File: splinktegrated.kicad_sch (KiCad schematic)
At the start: 51 parts, among them J1 USB_C_Receptacle_USB2.0, J10 Ribbon, J11 RJ9, J12 Conn_01x04_Female, J13 Conn_01x02_Female, J14 USB_C_Receptacle_USB2.0, J2 Conn_01x04_Female, J3 Conn_01x04_Female, J4 Conn_01x04_Female, J5 Conn_01x02, J6 RJ9, J7 trackball, J8 Ribbon, J9 RGB, SW1 SW_SPST, SW2 SW_SPST, U1 RP2040, U2 USBLC6-2P6, U3 XC6210B332MR-G, U4 USBLC6-2P6, U5 W25Q128JVS, Y1 Crystal_GND24

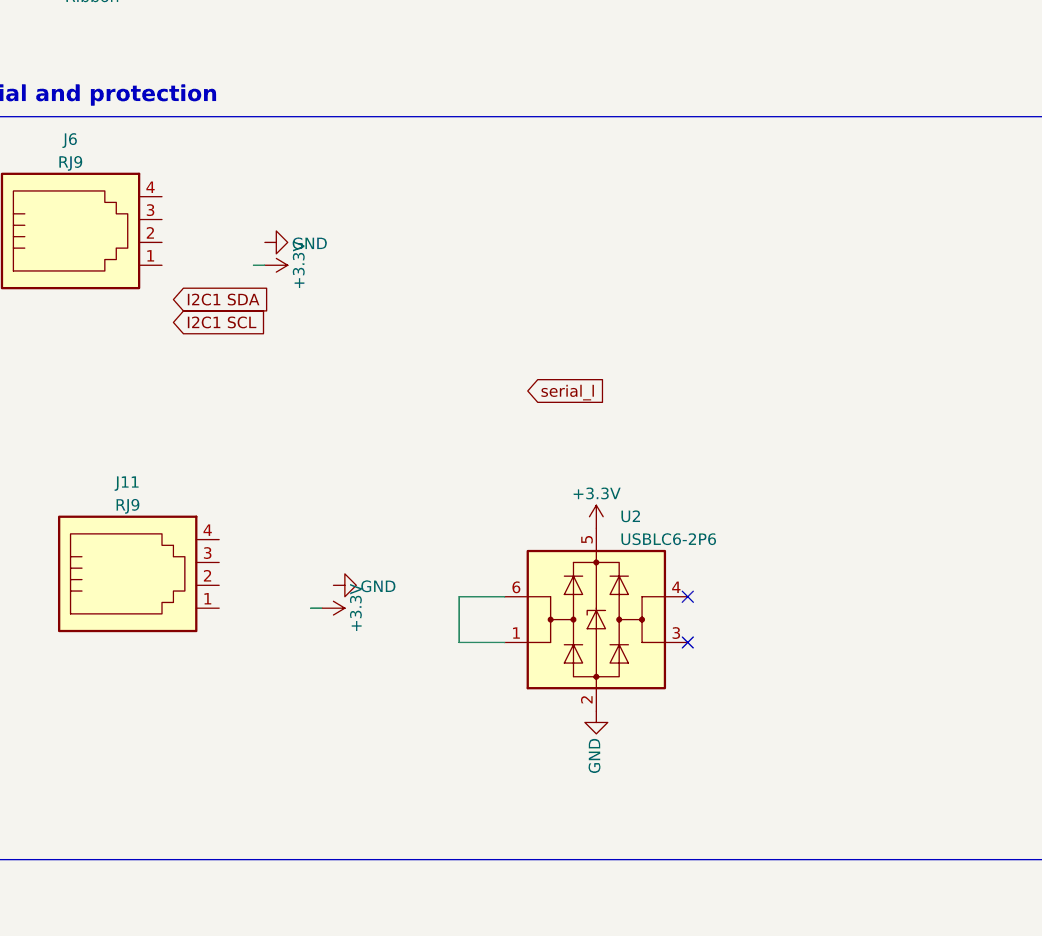
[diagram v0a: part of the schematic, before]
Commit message: minor changes
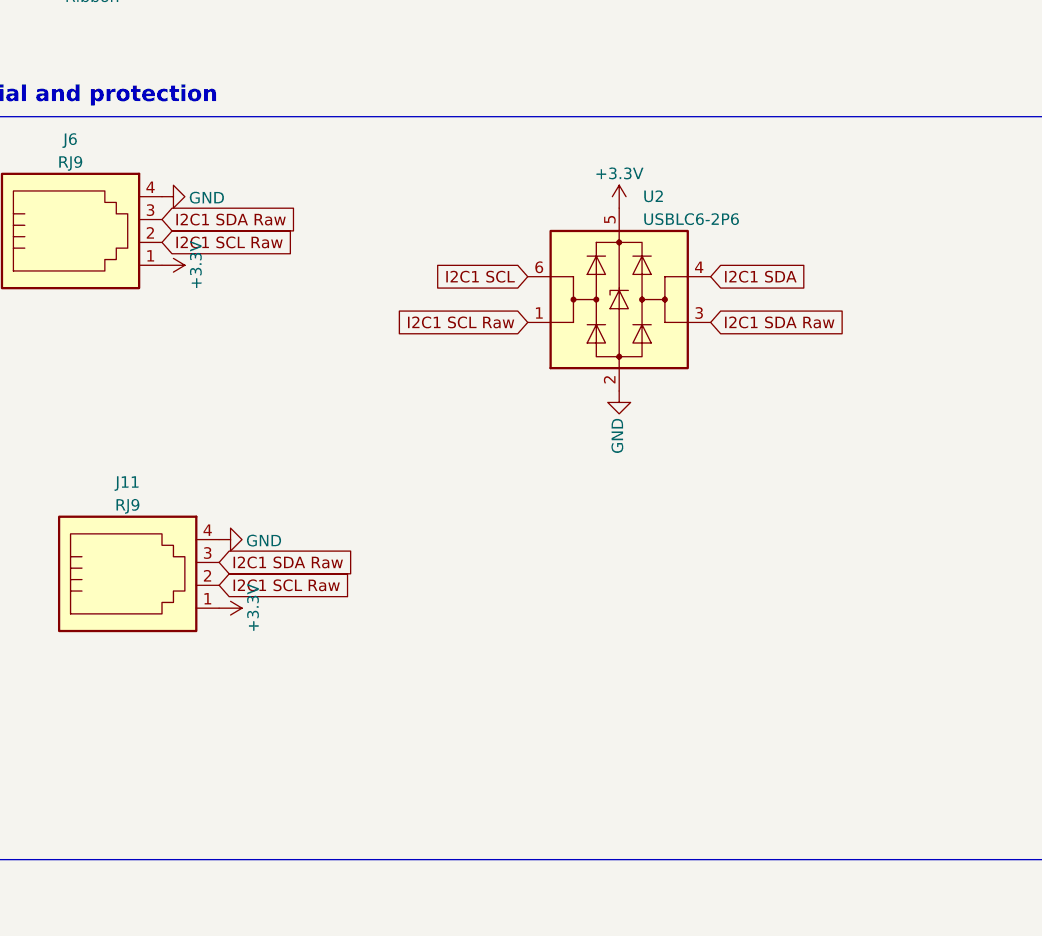
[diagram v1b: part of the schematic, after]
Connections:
- net +3V3: now also J11.1, J6.1
- net GND: now also J11.4, J6.4
- net I2C1 SCL: now also U2.6 (I/O1)
- net I2C1 SDA: now also U2.4 (I/O2)
- net I2C1 SCL Raw: now reaches J11.2
- net I2C1 SCL Raw: now also J6.2, U2.1 (I/O1)
- net I2C1 SDA Raw: now reaches J11.3
- net I2C1 SDA Raw: now also J6.3, U2.3 (I/O2)
- no-connect marks 14 -> 12
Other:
- moved on the sheet: U2

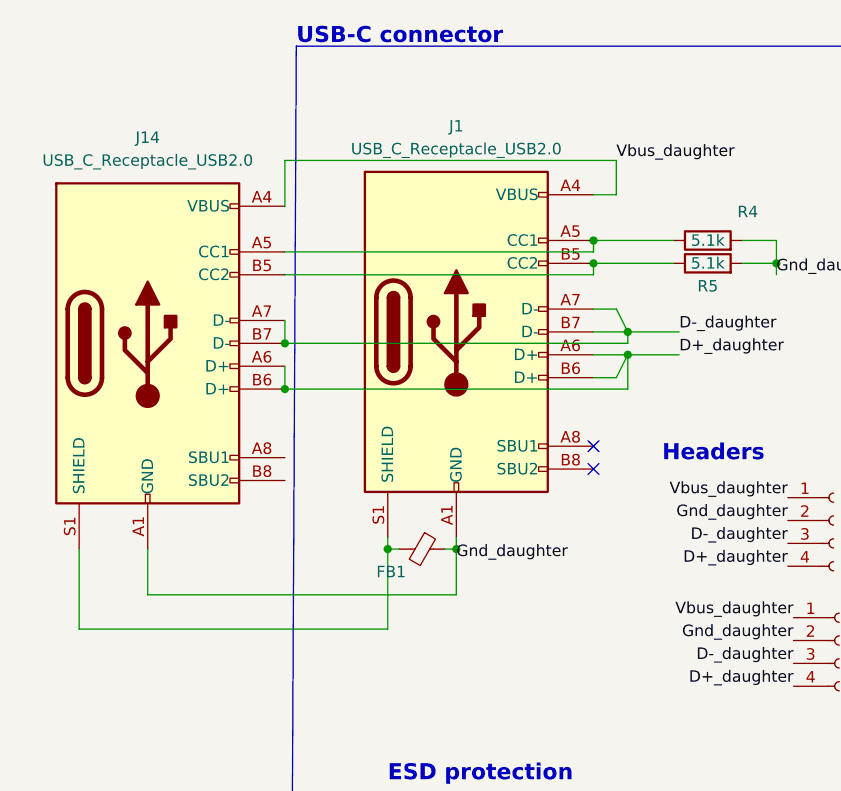
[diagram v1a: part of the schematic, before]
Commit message: major work done. outline finished
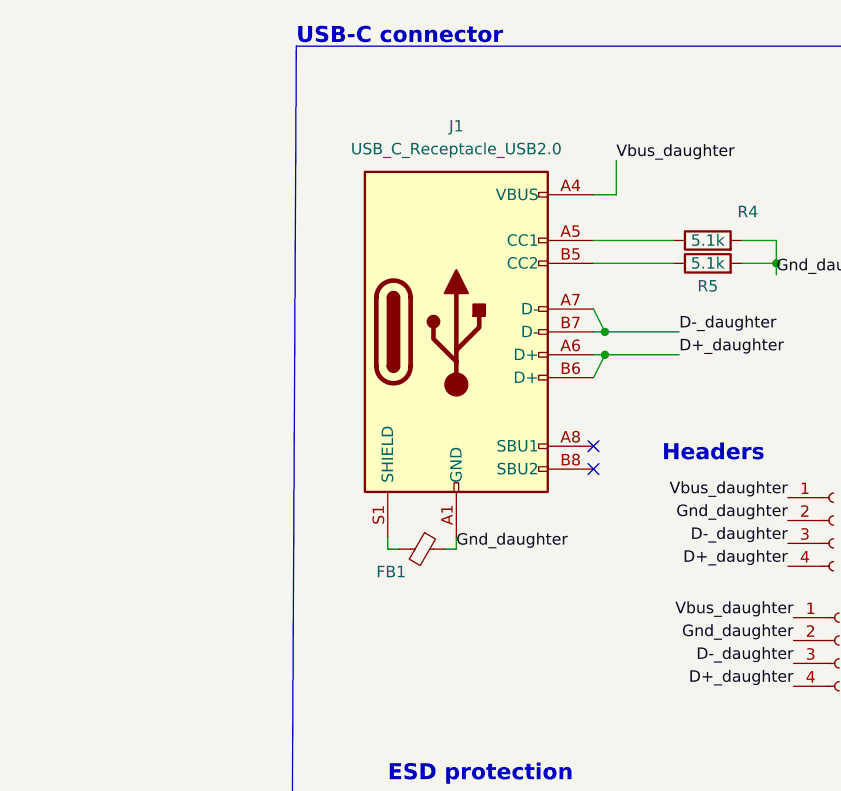
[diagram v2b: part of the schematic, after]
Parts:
- removed J14: USB_C_Receptacle_USB2.0, Connector_USB:USB_C_Receptacle_HRO_TYPE-C-31-M-12, symbol Connector:USB_C_Receptacle_USB2.0
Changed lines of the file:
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@@
     (company "bastardkb")
   )
-  (junction (at -123.19 54.61) (diameter 0) (color 0 0 0 0)
-  )
   (junction (at 46.99 127) (diameter 0) (color 0 0 0 0)
   )
@@
   (junction (at 154.94 38.1) (diameter 0) (color 0 0 0 0)
   )
+  (junction (at -87.63 50.8) (diameter 0) (color 0 0 0 0)
+  )
   (junction (at 162.56 38.1) (diameter 0) (color 0 0 0 0)
   )
@@
   (junction (at 40.005 172.72) (diameter 0) (color 0 0 0 0)
   )
-  (junction (at -85.09 48.26) (diameter 0) (color 0 0 0 0)
-  )
-  (junction (at -111.76 72.39) (diameter 0) (color 0 0 0 0)
-  )
   (junction (at 157.48 38.1) (diameter 0) (color 0 0 0 0)
   )
@@
   (junction (at 160.02 38.1) (diameter 0) (color 0 0 0 0)
   )
+  (junction (at -87.63 48.26) (diameter 0) (color 0 0 0 0)
+  )
   (junction (at 33.02 113.03) (diameter 0) (color 0 0 0 0)
   )
@@
   (junction (at 154.94 144.78) (diameter 0) (color 0 0 0 0)
   )
-  (junction (at -104.14 72.39) (diameter 0) (color 0 0 0 0)
-  )
   (junction (at 198.12 106.68) (diameter 0) (color 0 0 0 0)
   )
@@
   (junction (at -68.58 40.64) (diameter 0) (color 0 0 0 0)
   )
-  (junction (at -123.19 49.53) (diameter 0) (color 0 0 0 0)
-  )
   (junction (at 130.81 185.42) (diameter 0) (color 0 0 0 0)
   )
   (junction (at 97.79 106.68) (diameter 0) (color 0 0 0 0)
   )
-  (junction (at -88.9 38.1) (diameter 0) (color 0 0 0 0)
-  )
   (junction (at 33.02 115.57) (diameter 0) (color 0 0 0 0)
   )
-  (junction (at -85.09 50.8) (diameter 0) (color 0 0 0 0)
-  )
   (junction (at 243.84 119.38) (diameter 0) (color 0 0 0 0)
   )
   (junction (at 29.845 29.845) (diameter 0) (color 0 0 0 0)
-  )
-  (junction (at -88.9 40.64) (diameter 0) (color 0 0 0 0)
   )
   (junction (at 143.51 38.1) (diameter 0) (color 0 0 0 0)
@@
     (stroke (width 0) (type default))
   )
-  (wire (pts (xy -123.19 49.53) (xy -85.09 49.53))
-    (stroke (width 0) (type default))
-  )
-  (wire (pts (xy -123.19 41.91) (xy -88.9 41.91))
-    (stroke (width 0) (type default))
-  )
   (wire (pts (xy 101.6 175.26) (xy 110.49 175.26))
     (stroke (width 0) (type default))
@@
     (stroke (width 0) (type default))
   )
-  (wire (pts (xy -111.76 81.28) (xy -111.76 72.39))
-    (stroke (width 0) (type default))
-  )
-  (wire (pts (xy -88.9 50.8) (xy -85.09 50.8))
+  (wire (pts (xy -88.9 50.8) (xy -87.63 50.8))
     (stroke (width 0) (type default))
   )
@@
     (stroke (width 0) (type default))
   )
-  (wire (pts (xy -85.09 54.61) (xy -85.09 50.8))
-    (stroke (width 0) (type default))
-  )
   (wire (pts (xy 267.97 137.16) (xy 256.54 137.16))
     (stroke (width 0) (type default))
@@
     (stroke (width 0) (type default))
   )
-  (wire (pts (xy -138.43 72.39) (xy -138.43 77.47))
-    (stroke (width 0) (type default))
-  )
   (wire (pts (xy 48.895 29.845) (xy 52.705 29.845))
     (stroke (width 0) (type default))
@@
     (stroke (width 0) (type default))
   )
-  (wire (pts (xy -88.9 39.37) (xy -88.9 38.1))
-    (stroke (width 0) (type default))
-  )
-  (wire (pts (xy -85.09 48.26) (xy -88.9 48.26))
-    (stroke (width 0) (type default))
-  )
   (polyline (pts (xy -39.37 137.795) (xy -121.92 137.795))
     (stroke (width 0) (type default))
@@
     (stroke (width 0) (type default))
   )
-  (wire (pts (xy -88.9 45.72) (xy -86.36 45.72))
-    (stroke (width 0) (type default))
-  )
   (wire (pts (xy 93.98 90.17) (xy 93.98 104.14))
     (stroke (width 0) (type default))
@@
     (stroke (width 0) (type default))
   )
-  (wire (pts (xy -86.36 45.72) (xy -85.09 48.26))
+  (wire (pts (xy -88.9 45.72) (xy -87.63 48.26))
     (stroke (width 0) (type default))
   )
@@
     (stroke (width 0) (type default))
   )
-  (wire (pts (xy -123.19 29.21) (xy -86.36 29.21))
-    (stroke (width 0) (type default))
-  )
   (wire (pts (xy 182.88 109.22) (xy 191.77 109.22))
     (stroke (width 0) (type default))
@@
     (stroke (width 0) (type default))
   )
-  (wire (pts (xy -85.09 49.53) (xy -85.09 48.26))
-    (stroke (width 0) (type default))
-  )
   (wire (pts (xy 175.26 40.64) (xy 175.26 38.1))
     (stroke (width 0) (type default))
   )
-  (wire (pts (xy -146.05 72.39) (xy -146.05 81.28))
+  (wire (pts (xy -87.63 48.26) (xy -88.9 48.26))
     (stroke (width 0) (type default))
   )
@@
     (stroke (width 0) (type default))
   )
-  (wire (pts (xy -88.9 41.91) (xy -88.9 40.64))
-    (stroke (width 0) (type default))
-  )
   (wire (pts (xy 58.42 113.03) (xy 58.42 118.11))
     (stroke (width 0) (type default))
@@
     (stroke (width 0) (type default))
   )
-  (wire (pts (xy -123.19 52.07) (xy -123.19 54.61))
-    (stroke (width 0) (type default))
-  )
-  (wire (pts (xy -123.19 54.61) (xy -85.09 54.61))
-    (stroke (width 0) (type default))
-  )
   (wire (pts (xy 148.59 175.26) (xy 157.48 175.26))
     (stroke (width 0) (type default))
@@
     (stroke (width 0) (type default))
   )
-  (wire (pts (xy -146.05 81.28) (xy -111.76 81.28))
-    (stroke (width 0) (type default))
-  )
   (wire (pts (xy 82.55 184.15) (xy 82.55 186.69))
     (stroke (width 0) (type default))
@@
     (stroke (width 0) (type default))
   )
-  (wire (pts (xy -123.19 39.37) (xy -88.9 39.37))
-    (stroke (width 0) (type default))
-  )
   (wire (pts (xy 97.79 105.41) (xy 97.79 106.68))
     (stroke (width 0) (type default))
@@
     (stroke (width 0) (type default))
   )
-  (wire (pts (xy -123.19 34.29) (xy -123.19 29.21))
-    (stroke (width 0) (type default))
-  )
   (wire (pts (xy 97.79 96.52) (xy 101.6 96.52))
     (stroke (width 0) (type default))
@@
     (stroke (width 0) (type default))
   )
-  (wire (pts (xy -138.43 77.47) (xy -104.14 77.47))
-    (stroke (width 0) (type default))
-  )
   (wire (pts (xy 91.44 184.15) (xy 91.44 186.69))
     (stroke (width 0) (type default))
@@
     (stroke (width 0) (type default))
   )
-  (wire (pts (xy -104.14 72.39) (xy -104.14 77.47))
-    (stroke (width 0) (type default))
-  )
   (polyline (pts (xy 77.47 194.31) (xy 172.72 194.31))
     (stroke (width 0) (type default))
@@
     (stroke (width 0) (type default))
   )
+  (wire (pts (xy -87.63 50.8) (xy -79.375 50.8))
+    (stroke (width 0) (type default))
+  )
   (wire (pts (xy 111.76 83.82) (xy 116.84 83.82))
     (stroke (width 0) (type default))
@@
     (stroke (width 0) (type default))
   )
-  (wire (pts (xy -85.09 50.8) (xy -86.36 53.34))
+  (wire (pts (xy -87.63 50.8) (xy -88.9 53.34))
     (stroke (width 0) (type default))
   )
@@
     (stroke (width 0) (type default))
   )
-  (wire (pts (xy -85.09 48.26) (xy -79.375 48.26))
-    (stroke (width 0) (type default))
-  )
   (wire (pts (xy 138.43 40.64) (xy 138.43 38.1))
     (stroke (width 0) (type default))
@@
     (stroke (width 0) (type default))
   )
-  (wire (pts (xy -123.19 46.99) (xy -123.19 49.53))
-    (stroke (width 0) (type default))
-  )
   (wire (pts (xy 182.88 134.62) (xy 191.77 134.62))
     (stroke (width 0) (type default))
@@
     (stroke (width 0) (type default))
   )
-  (wire (pts (xy -86.36 53.34) (xy -88.9 53.34))
-    (stroke (width 0) (type default))
-  )
   (wire (pts (xy 110.49 176.53) (xy 110.49 175.26))
     (stroke (width 0) (type default))
   )
-  (wire (pts (xy -85.09 50.8) (xy -79.375 50.8))
-    (stroke (width 0) (type default))
-  )
   (wire (pts (xy 157.48 184.15) (xy 157.48 185.42))
     (stroke (width 0) (type default))
@@
   )
   (wire (pts (xy 182.88 71.12) (xy 191.77 71.12))
+    (stroke (width 0) (type default))
+  )
+  (wire (pts (xy -87.63 48.26) (xy -79.375 48.26))
     (stroke (width 0) (type default))
   )
@@
     (effects (font (size 1.27 1.27)) (justify left bottom))
   )
-  (label "Gnd_daughter" (at -104.14 73.66 0) (fields_autoplaced)
+  (label "Gnd_daughter" (at -104.14 72.39 0) (fields_autoplaced)
     (effects (font (size 1.27 1.27)) (justify left bottom))
   )
@@
         )
       )
-    )
-  )
-  (symbol (lib_id "Connector:USB_C_Receptacle_USB2.0") (at -138.43 49.53 0) (unit 1)
-    (in_bom yes) (on_board yes) (dnp no) (fields_autoplaced)
-    (property "Reference" "J14" (at -138.43 26.67 0)
-      (effects (font (size 1.27 1.27)))
-    )
-    (property "Value" "USB_C_Receptacle_USB2.0" (at -138.43 29.21 0)
-      (effects (font (size 1.27 1.27)))
-    )
-    (property "Footprint" "Connector_USB:USB_C_Receptacle_HRO_TYPE-C-31-M-12" (at -134.62 49.53 0)
-      (effects (font (size 1.27 1.27)) hide)
-    )
-    (property "Datasheet" "https://www.usb.org/sites/default/files/documents/usb_type-c.zip" (at -134.62 49.53 0)
-      (effects (font (size 1.27 1.27)) hide)
-    )
-    (property "LCSC" "C223907" (at -138.43 49.53 0)
-      (effects (font (size 1.27 1.27)) hide)
-    )
-    (pin "A1")
-    (pin "A12")
-    (pin "A4")
-    (pin "A5")
-    (pin "A6")
-    (pin "A7")
-    (pin "A8")
-    (pin "A9")
-    (pin "B1")
-    (pin "B12")
-    (pin "B4")
-    (pin "B5")
-    (pin "B6")
-    (pin "B7")
-    (pin "B8")
-    (pin "B9")
-    (pin "S1")
-    (instances
-      (project "splinktegrated"
-        (path "/7353e96a-343a-4876-b497-b1d205a14d97"
-          (reference "J14") (unit 1)
-        )
-      )
